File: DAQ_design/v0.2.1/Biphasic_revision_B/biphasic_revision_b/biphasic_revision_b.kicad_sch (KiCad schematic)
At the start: 19 parts, among them Q1 BC549, Q2 IRF9540N, Q3 IRF540N, Q4 BC549, Q5 IRF9540N, Q6 IRF540N, U1 ADS1115IDGS

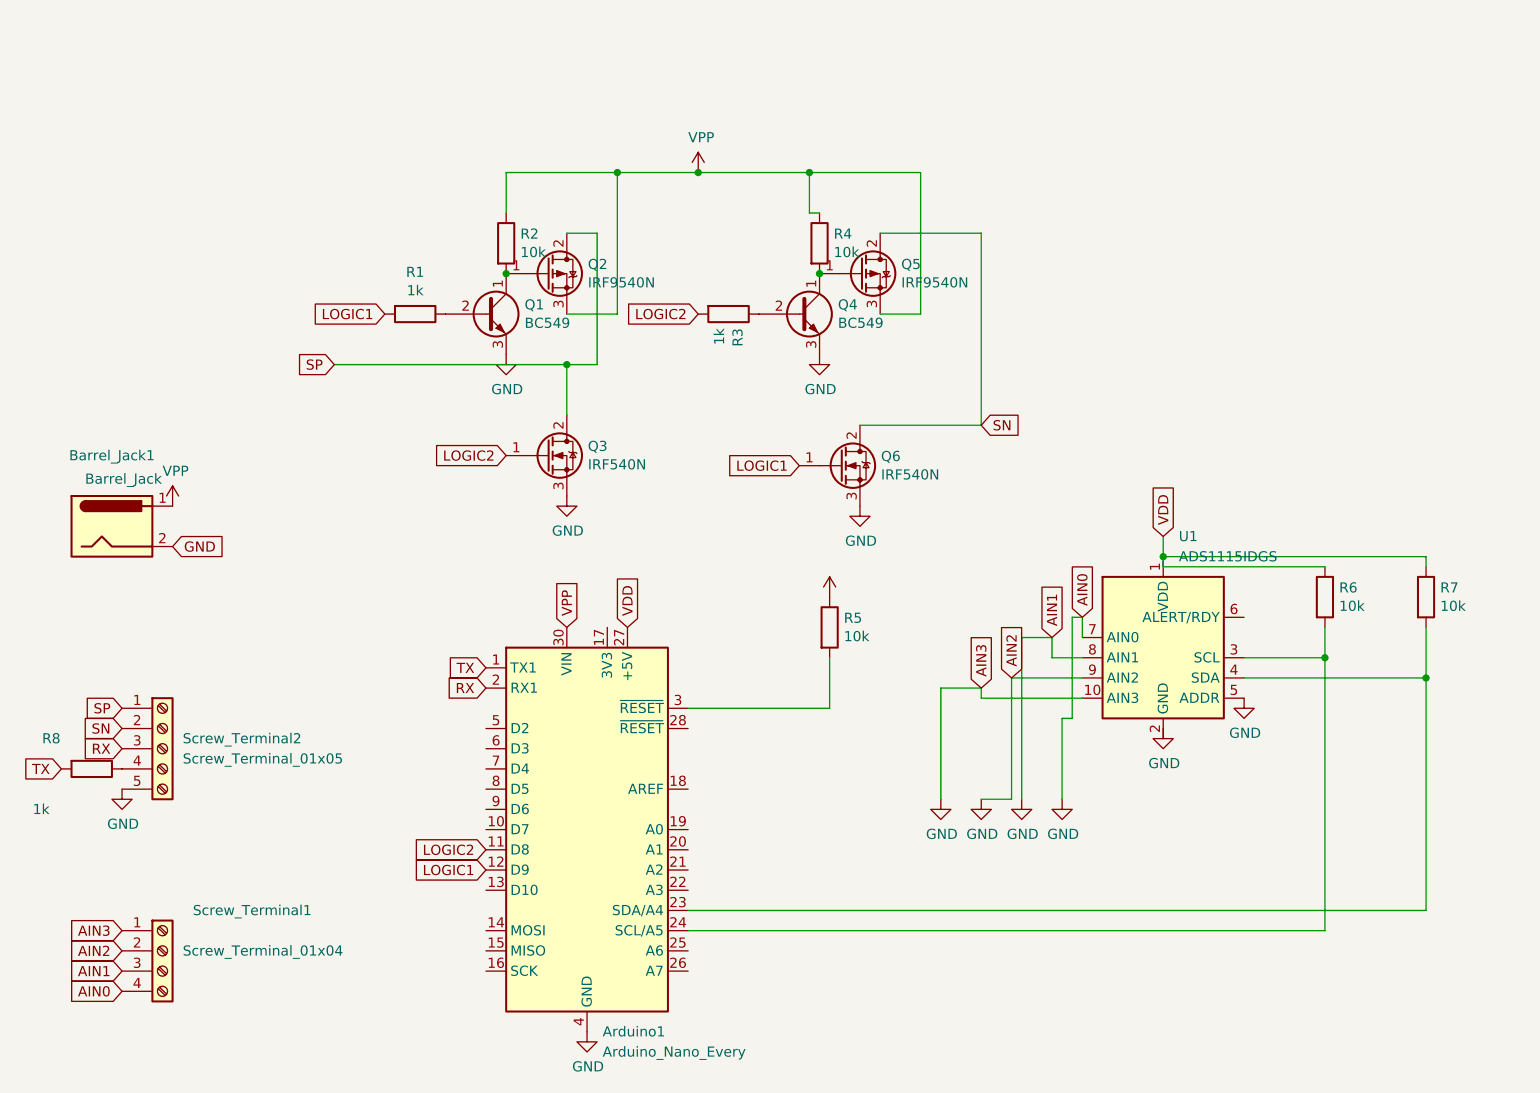
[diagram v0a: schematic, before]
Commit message: naming
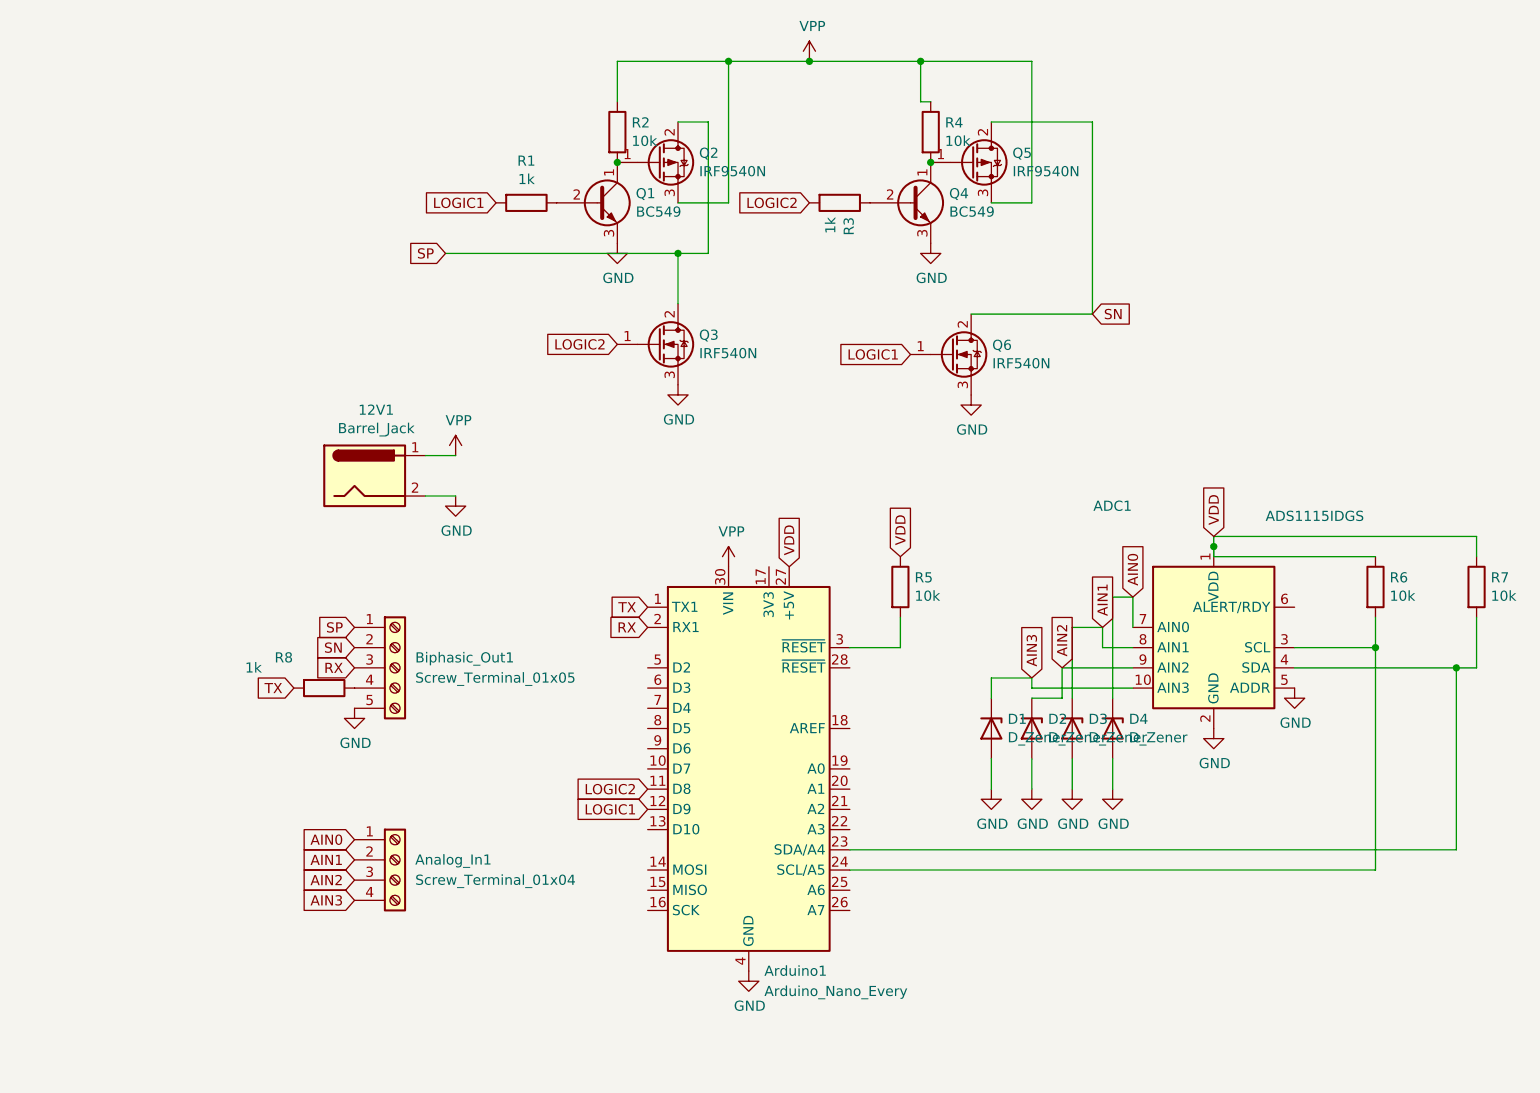
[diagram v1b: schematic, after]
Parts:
- removed Screw_Terminal1: Screw_Terminal_01x04, TerminalBlock:TerminalBlock_bornier-4_P5.08mm, symbol Connector:Screw_Terminal_01x04
- removed Screw_Terminal2: Screw_Terminal_01x05, TerminalBlock:TerminalBlock_bornier-5_P5.08mm, symbol Connector:Screw_Terminal_01x05
- removed U1: ADS1115IDGS, ads1115module:Adafruit_ADS1115, symbol Analog_ADC:ADS1115IDGS
- added ADC1: ADS1115IDGS, ads1115module:Adafruit_ADS1115, symbol Analog_ADC:ADS1115IDGS
- added Analog_In1: Screw_Terminal_01x04, TerminalBlock:TerminalBlock_bornier-4_P5.08mm, symbol Connector:Screw_Terminal_01x04
- added Biphasic_Out1: Screw_Terminal_01x05, TerminalBlock:TerminalBlock_bornier-5_P5.08mm, symbol Connector:Screw_Terminal_01x05
- added D1, D2, D3, D4: D_Zener, Diode_THT:D_DO-35_SOD27_P7.62mm_Horizontal, symbol Device:D_Zener
- Arduino1: footprint Module:Arduino_Nano_WithMountingHoles -> Module:Arduino_Nano
- R1, R2, R3, R4, R5, R6, R7, R8: footprint Resistor_SMD:R_0603_1608Metric -> Resistor_SMD:R_1206_3216Metric
- renumbered Barrel_Jack1 to 12V1
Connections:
- net GND: now also ADC1.2 (GND), ADC1.5 (ADDR), Biphasic_Out1.5 (Pin_5), D1.2 (A), D2.2 (A), D3.2 (A), D4.2 (A)
- net RX: now also Biphasic_Out1.3 (Pin_3)
- net SN: now also Biphasic_Out1.2 (Pin_2)
- net SP: now also Biphasic_Out1.1 (Pin_1)
- net VDD: now also ADC1.1 (VDD)
- net at Arduino1.24 (SCL/A5), R6.2: now also ADC1.3 (SCL)
- net at Arduino1.23 (SDA/A4), R7.2: now also ADC1.4 (SDA)
- net at R8.1: now also Biphasic_Out1.4 (Pin_4)
- new net AIN0: ADC1.7 (AIN0), Analog_In1.1 (Pin_1), D4.1 (K)
- new net AIN1: ADC1.8 (AIN1), Analog_In1.2 (Pin_2), D3.1 (K)
- new net AIN2: ADC1.9 (AIN2), Analog_In1.3 (Pin_3), D2.1 (K)
- new net AIN3: ADC1.10 (AIN3), Analog_In1.4 (Pin_4), D1.1 (K)
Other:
- moved on the sheet: 12V1, Q1, Q2, Q3, Q4, Q5, Q6, R1, R2, R3, R4, R5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
